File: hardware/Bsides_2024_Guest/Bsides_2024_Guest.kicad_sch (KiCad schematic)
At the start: 44 parts, among them J1 Conn_02x03_Odd_Even, J2 Battery, J3 Battery, J4 OLED, J5 Conn_01x05, J6 Conn_01x05, P1 USB_C_Plug_USB2.0, Q1 DMG3415U-7, SW1 ON, SW2 RESET, SW3 BOOT, SW4 RESET, SW6 RESET, U1 ESP32-C6-WROOM-1U-N4, U2 AP2112K-3.3

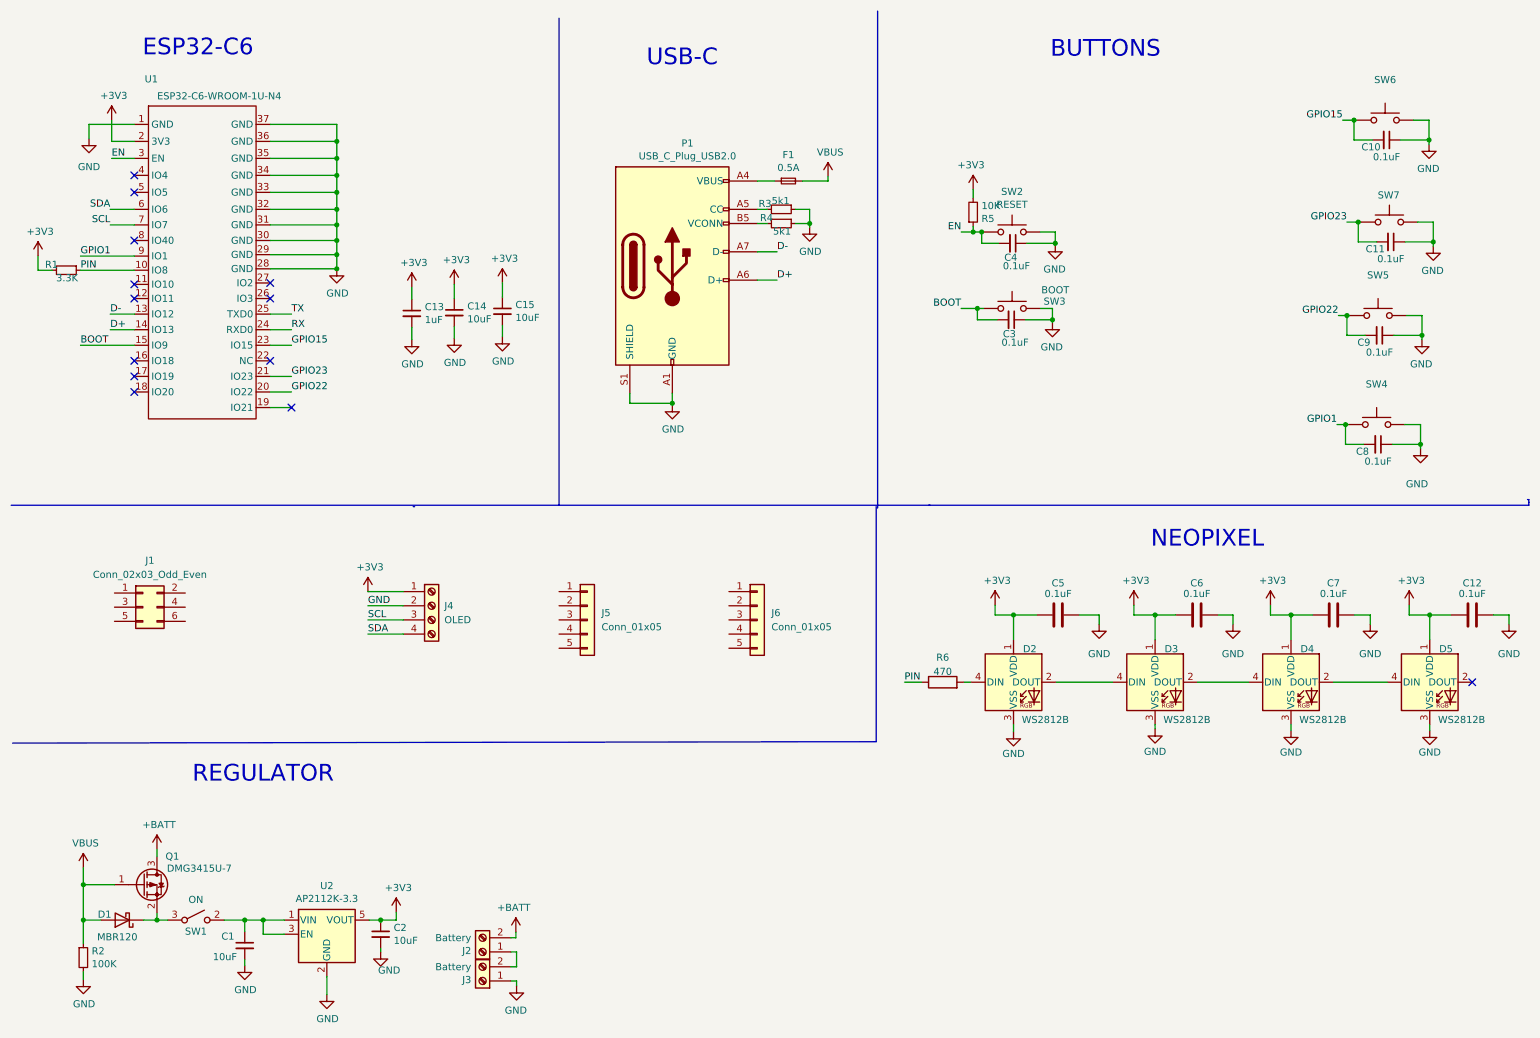
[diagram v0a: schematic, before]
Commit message: feat(Hw): Update PCB
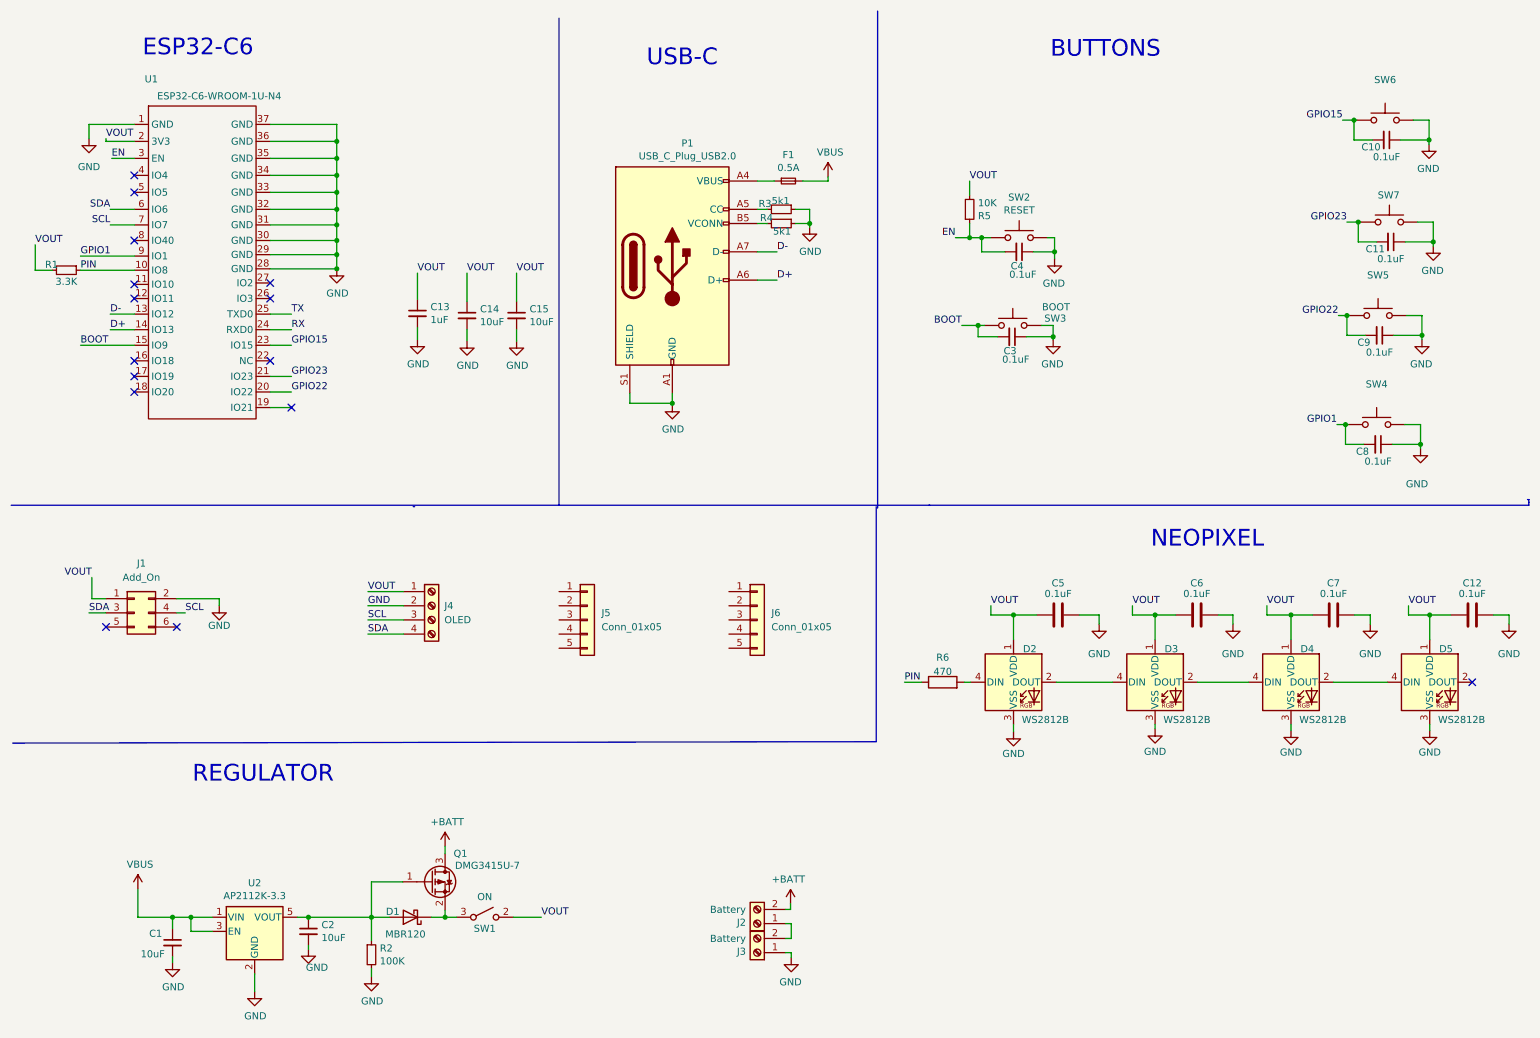
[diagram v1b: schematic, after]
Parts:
- J1: value Conn_02x03_Odd_Even -> Add_On
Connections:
- net GND: now also J1.2 (Pin_2)
- net SCL: now also J1.4 (Pin_4)
- net SDA: now also J1.3 (Pin_3)
- net VBUS: now also C1.1, U2.1 (VIN), U2.3 (EN); no longer D1.2 (A), Q1.1 (G), R2.1
- net VOUT: now reaches J1.1 (Pin_1)
- net VOUT: now also C12.2, C13.1, C14.1, C15.1, C5.2, C6.2, C7.2, D2.1 (VDD), D3.1 (VDD), D4.1 (VDD), D5.1 (VDD), J4.1 (Pin_1), R1.2, R5.2, SW1.2 (B), U1.2 (3V3)
- removed net +3V3: C12.2, C13.1, C14.1, C15.1, C2.1, C5.2, C6.2, C7.2, D2.1 (VDD), D3.1 (VDD), D4.1 (VDD), D5.1 (VDD), J4.1 (Pin_1), R1.2, R5.2, U1.2 (3V3), U2.5 (VOUT)
- new net: C2.1, D1.2 (A), Q1.1 (G), R2.1, U2.5 (VOUT)
- no-connect marks 13 -> 15
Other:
- moved on the sheet: C1, C13, C14, C15, C2, C3, C4, D1, J1, J2, J3, Q1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
